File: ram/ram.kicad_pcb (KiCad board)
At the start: 4 copper layers, 102.4 x 40.3 mm, 7 parts, among them J2 Conn_01x03, U1 IS66WVE4M16EBLL-70BLI, U3 74LVC2G00

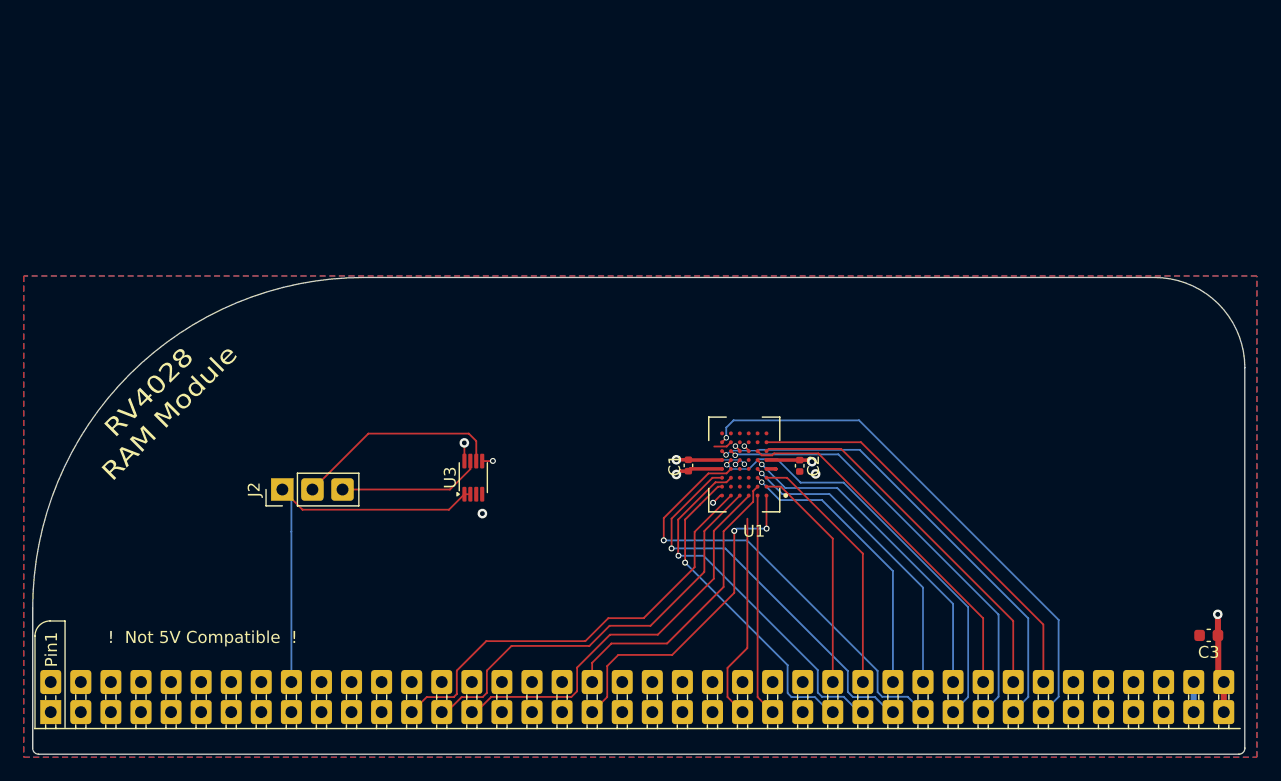
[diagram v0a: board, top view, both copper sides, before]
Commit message: RAM board attempt 2
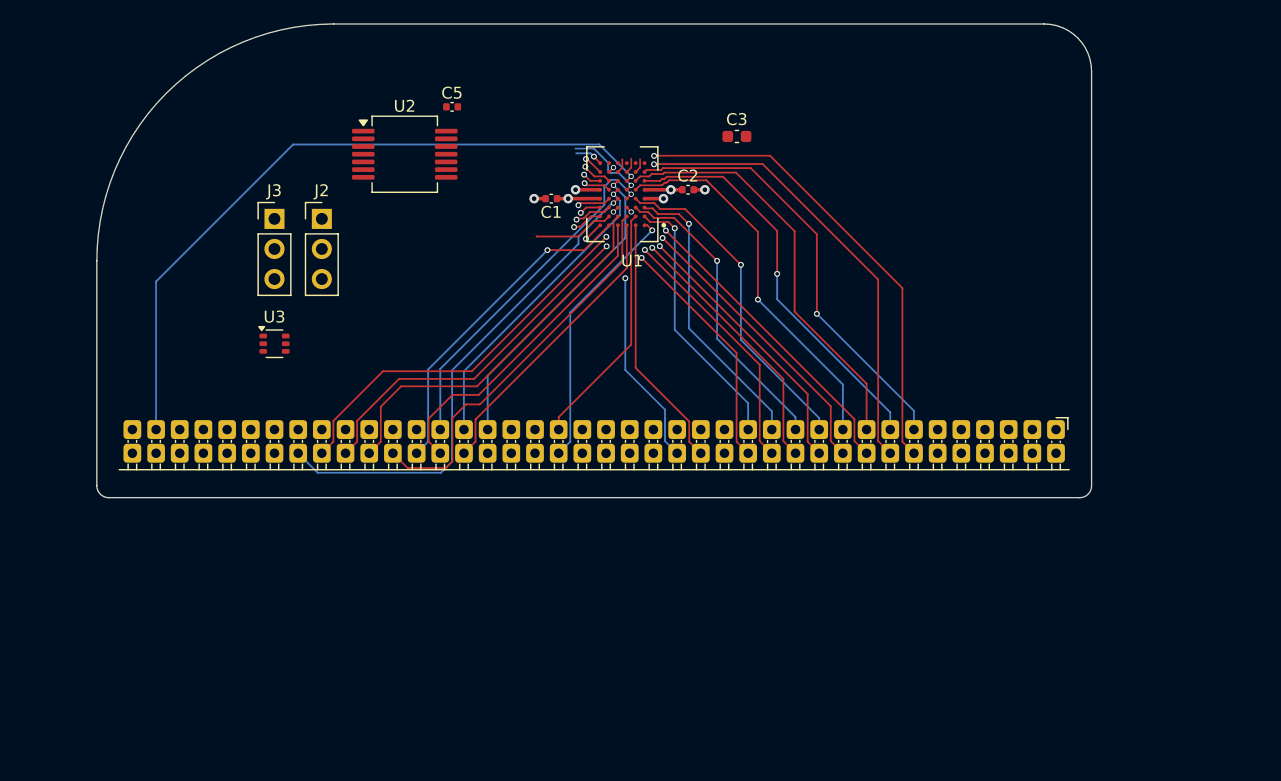
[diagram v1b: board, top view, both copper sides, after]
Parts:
- added C5: 100n, Capacitor_SMD:C_0402_1005Metric, F.Cu at (120.0, 67.0)
- added J3: Conn_01x03, Connector_PinHeader_2.54mm:PinHeader_1x03_P2.54mm_Vertical, F.Cu at (105.0, 76.5)
- added U2: 74LVC32, Package_SO:SSOP-14_5.3x6.2mm_P0.65mm, F.Cu at (116.0, 71.0)
- J1: footprint RV4028:ModuleHeader -> RV4028:Module_2mm
- U3: value 74LVC2G00 -> 74LVC2G04; footprint Package_SO:VSSOP-8_2.3x2mm_P0.5mm -> Package_TO_SOT_SMD:SOT-363_SC-70-6
- moved C3 58.0 mm to (144.1, 69.5), turned to 0 degrees
- moved C1 25.3 mm to (128.4, 74.8), turned to 180 degrees
- moved C2 25.1 mm to (139.9, 74.0), turned to 0 degrees
- moved U1 25.0 mm to (134.4, 74.4)
- moved J2 23.1 mm to (109.0, 76.5), turned to 0 degrees
- moved J1 22.3 mm to (132.0, 95.8)
- moved U3 20.2 mm to (105.0, 87.0), turned to 0 degrees
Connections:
- J1 pad 18: unconnected-(J1-PWR-Pad18) -> +3V3
- J1 pad 23: unconnected-(J1-~{REQ}-Pad23) -> /~{REQ}
- J1 pad 40: +3V3 -> unconnected-(J1-+5V-Pad40)
- J1 pad 48: unconnected-(J1-A24-Pad48) -> /A24
- J1 pad 58: unconnected-(J1-PWR-Pad58) -> +3V3
- J1 pad 60: unconnected-(J1-~{RST2}-Pad60) -> GND
- J1 pad 61: unconnected-(J1-CLK2-Pad61) -> GND
- J1 pad 63: /LO_ADDR -> /~{LO_ADDR}
- J1 pad 66: unconnected-(J1-SPARE1-Pad66) -> GND
- J1 pad 80: +3V3 -> unconnected-(J1-+5V-Pad80)
- U3 pad 2: /A23 -> GND
- U3 pad 3: /~{CE} -> /A24
- U3 pad 4: GND -> /~{A24}
- U3 pad 5: /LO_ADDR -> +3V3
- U3 pad 6: Net-(J2-Pin_2) -> /~{A23}
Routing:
- net /A15: track 0.58 -> 59.1 mm
- net /A8: track 0.00 -> 42.1 mm, vias 0 -> 1
- net /A7: track 0.00 -> 35.5 mm, vias 0 -> 2
- net /A6: track 0.00 -> 34.6 mm, vias 0 -> 2
- net /A4: track 0.00 -> 33.2 mm
- net /A23: track 32.6 -> 0.00 mm
- net /A5: track 0.00 -> 32.4 mm
- net /A18: track 0.00 -> 29.8 mm, vias 0 -> 1
- net /A16: track 0.58 -> 26.4 mm
- net /A17: track 0.54 -> 26.1 mm
- net Net-(J2-Pin_2): track 17.7 -> 0.00 mm
- net /~{A23}: track 12.2 -> 0.00 mm
- net +3V3: track 19.0 -> 8.54 mm, vias 5 -> 3
- net /A3: track 37.4 -> 27.8 mm, vias 0 -> 1
- net /~{WE}: track 19.1 -> 28.7 mm, vias 0 -> 2
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- removed copper zone on B.Cu, net GND
- removed copper zone on F.Cu, net GND
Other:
- board size 102.4 x 40.3 mm -> 84 x 40 mm
- board text removed: "! Not 5V Compatible !"
- board text removed: "RV4028 RAM"
- board text removed: "RV4028 RAM Module"
